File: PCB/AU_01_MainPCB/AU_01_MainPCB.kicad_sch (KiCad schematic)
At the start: 0 parts

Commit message: Created USB-C Schematic
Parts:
- added C1, C38, C39, C46, C47, C48, C49, C50, C51, C53, C54, C55, C56, C57, C58: 100nF, symbol Device:C
- added C2: 1uF, symbol Device:C
- added C40, C42, C45: 10uF, symbol Device:C_Polarized
- added C41: 10uF (Tantalum), symbol Device:C_Polarized
- added C52: 150uF, symbol Device:C_Polarized
- added CR1: SP3010-04UTG, UDFEN-10_MO229_LTF, symbol SP3010-04UTG:SP3010-04UTG
- added D1: SMAJ33CA, Diode_SMD:D_SMA, symbol Diode:SMAJ33CA
- added D11: D, symbol Device:D
- added J1: SS-53200-001, SS-53200-001:STEWART_SS-53200-001, symbol SS-53200-001:SS-53200-001
- added J6: 1-2199230-6, 1-2199230-6:TE_1-2199230-6, symbol 1-2199230-6:1-2199230-6
- added R17: 10k, symbol Device:R
- added U1: (no value), symbol Firefly_I-CORE3576Q38:I-CORE3576Q38
- added U18: SSP7903P12FR, Package_TO_SOT_SMD:SOT-223-3_TabPin2, symbol Regulator_Linear:LM317_SOT-223
- added U19: AMS1086CM3.3, TO-263DD_M_ADS, symbol AMS1086CM-3.3:AMS1086CM3.3
- added U2, U3: TPD4E02B04DQA, Package_SON:USON-10_2.5x1.0mm_P0.5mm, symbol Power_Protection:TPD4E02B04DQA
- added VR1: LM1085ISX-5.0_NOPB, LM1085ISX-5.0_NOPB:TO254P1435X464-4N, symbol LM1085ISX-5.0/NOPB:LM1085ISX-5.0_NOPB
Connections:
- new net: C49.2, U1.70 (USB3_OTG0_SSRX2N)
- new net: C51.2, U1.74 (USB3_OTG0_SSTX2P)
- new net: C46.2, U1.64 (USB3_OTG0_SSTX1P)
- new net: C53.1, U1.29 (PCIE0_REFCLKN_(OUTPUT))
- new net: C53.2, J6.53
- new net: J6.54, U1.138 (PCIE0_WAKEN_M1)
- new net: J6.52, U1.142 (PCIE0_CLKREQN_M1)
- new net: CR1.1, CR1.10, J1.15 (SCL), U1.15 (PWM2_CH0_M1)
- new net: R17.1, U1.16 (USB2_OTG0_VBUSDET)
- new net: CR1.4, CR1.7, J1.19 (HOT_PLUG_DETECT), U1.17 (PWM0_CH1_M1)
- new net: CR1.2, CR1.9, J1.16 (SDA), U1.21 (PWM2_CH1_M1)
- new net: C54.1, U1.31 (PCIE0_REFCLKP_(OUTPUT))
- new net: C55.1, U1.33 (PCIE0_RXN)
- new net: C56.1, U1.35 (PCIE0_RXP)
- new net: C57.1, U1.37 (PCIE0_TXN)
- new net: C58.1, U1.39 (PCIE0_TXP)
- new net: C38.2, U1.60 (USB3_OTG0_SSRX1P)
- new net: C39.2, U1.62 (USB3_OTG0_SSRX1N)
- new net: C47.2, U1.66 (USB3_OTG0_SSTX1N)
- new net: C48.2, U1.68 (USB3_OTG0_SSRX2P)
- new net: C50.2, U1.72 (USB3_OTG0_SSTX2N)
- new net: J1.12 (DATA3-), U1.83 (HDMI_TX_D3N), U2.5 (IO4), U2.6 (NC)
- new net: J1.10 (DATA3+), U1.85 (HDMI_TX_D3P), U2.4 (IO3), U2.7 (NC)
- new net: J1.9 (DATA0-), U1.87 (HDMI_TX_D0N), U2.2 (IO2), U2.9 (NC)
- new net: J1.7 (DATA0+), U1.89 (HDMI_TX_D0P), U2.1 (IO1), U2.10 (NC)
- new net: J1.6 (DATA1-), U1.91 (HDMI_TX_D1N), U3.5 (IO4), U3.6 (NC)
- new net: J1.4 (DATA1+), U1.93 (HDMI_TX_D1P), U3.4 (IO3), U3.7 (NC)
- new net: J1.3 (DATA2-), U1.95 (HDMI_TX_D2N), U3.2 (IO2), U3.9 (NC)
- new net: J1.1 (DATA2+), U1.97 (HDMI_TX_D2P), U3.1 (IO1), U3.10 (NC)
- new net: C56.2, J6.43
- new net: C55.2, J6.41
- new net: C58.2, J6.49
- new net: C57.2, J6.47
- new net: C54.2, J6.55
- new net 12V: C45.1, U18.2 (VO)
- new net 3V3_HIPWR: C52.1, D11.2 (A), J6.12, J6.14, J6.16, J6.18, J6.2, J6.4, J6.70, J6.72, J6.74, U19.2 (VOUT), U19.4 (OUTPUT)
- new net 3V3_O: U1.125 (VCC_3V3_S3_（OUTPUT）), U1.127 (VCC_3V3_S3_（OUTPUT）)
- new net GND: C1.2, C2.2, C40.2, C41.2, C42.2, C45.2, C52.2, CR1.3, CR1.5, CR1.6, CR1.8, D1.1 (A1), J1.11 (DATA3_SHIELD), J1.17 (DDC/CEC_GND), J1.2 (DATA2_SHIELD), J1.5 (DATA1_SHIELD), J1.8 (DATA0_SHIELD), J1.SH1 (SHIELD), J1.SH2 (SHIELD), J1.SH3 (SHIELD), J1.SH4 (SHIELD), J6.1, J6.15, J6.21, J6.27, J6.3, J6.33, J6.39, J6.45, J6.51, J6.57, J6.71, J6.73, J6.75, J6.9, J6.S1 (SHIELD), J6.S2 (SHIELD), R17.2, U1.110 (GND), U1.111 (GND), U1.112 (GND), U1.113 (GND), U1.114 (GND), U1.115 (GND), U1.116 (GND), U1.117 (GND), U1.122 (GND), U1.132 (GND), U1.143 (GND), U1.146 (GND), U1.157 (GND), U1.168 (GND), U1.169 (GND), U1.2 (GND), U1.27 (GND), U1.41 (GND), U1.44 (GND), U1.54 (GND), U1.55 (GND), U1.76 (GND), U1.77 (GND), U1.99 (GND), U18.1 (ADJ), U19.1 (GND), U2.3 (G), U2.8 (G), U3.3 (G), U3.8 (G), VR1.1 (ADJ/GND)
- new net SCL_6: U1.25 (PWM2_CH2_M1)
- new net SDA_6: U1.23 (PWM2_CH3_M1)
- new net SYS_5V: C1.1, C2.1, C41.1, D1.2 (A2), D11.1 (K), J1.18 (+5V), U1.101 (VCC5V0_SYS_S5), U1.102 (VCC5V0_SYS_S5), U1.103 (VCC5V0_SYS_S5), U1.104 (VCC5V0_SYS_S5), U1.105 (VCC5V0_SYS_S5), U1.106 (VCC5V0_SYS_S5), U1.107 (VCC5V0_SYS_S5), U1.108 (VCC5V0_SYS_S5), U1.109 (VCC5V0_SYS_S5), U19.3 (VIN), VR1.2 (OUTPUT_2), VR1.4 (OUTPUT_4)
- new net USBC0_DN: U1.48 (USB2_OTG1_DM)
- new net USBC0_DP: U1.46 (USB2_OTG1_DP)
- new net USBC1_DN_O: U1.52 (USB2_OTG0_DM)
- new net USBC1_DP_O: U1.50 (USB2_OTG0_DP)
- new net USBC1_SSRX1N: C47.1
- new net USBC1_SSRX1P: C46.1
- new net USBC1_SSRX2N: C50.1
- new net USBC1_SSRX2P: C51.1
- new net USBC1_SSTX1N: C39.1
- new net USBC1_SSTX1P: C38.1
- new net USBC1_SSTX2N: C49.1
- new net USBC1_SSTX2P: C48.1
- new net USBC1_SW_EN: U1.6 (CAN1_TX_M2)
- new net USBC_1_INT: U1.4 (SPDIF_RX0_M0)
- new net VSYS: C40.1, C42.1, U18.3 (VI), VR1.3 (INPUT)
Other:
- added sheet AU_01 Audio System (AU_01_AudioSystem.kicad_sch)
- added sheet AU_01 Battery Circuit (AU_01_BatteryCircuit.kicad_sch)
- added sheet AU_01 USB-C Ports (AU_01_USBC_Ports.kicad_sch)

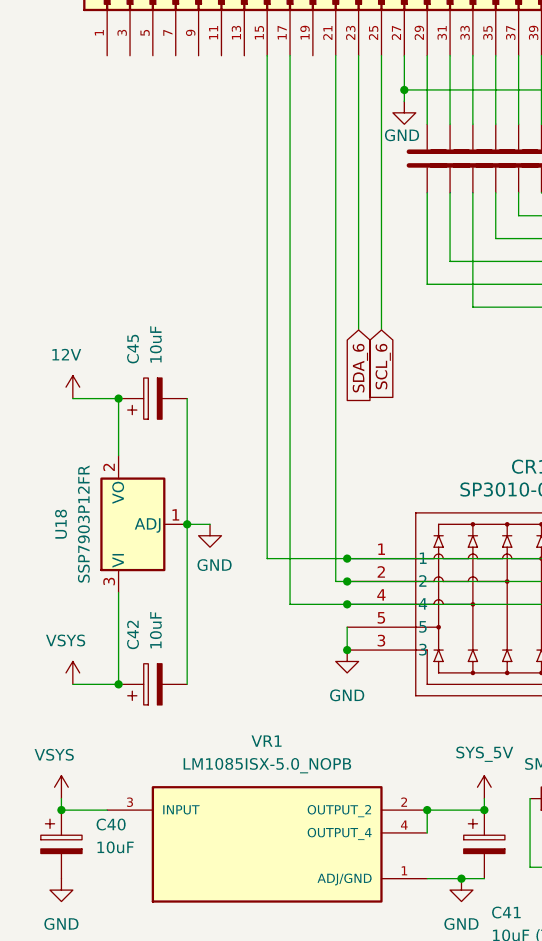
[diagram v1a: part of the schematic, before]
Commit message: Audio, Battery Schematic, added Journal
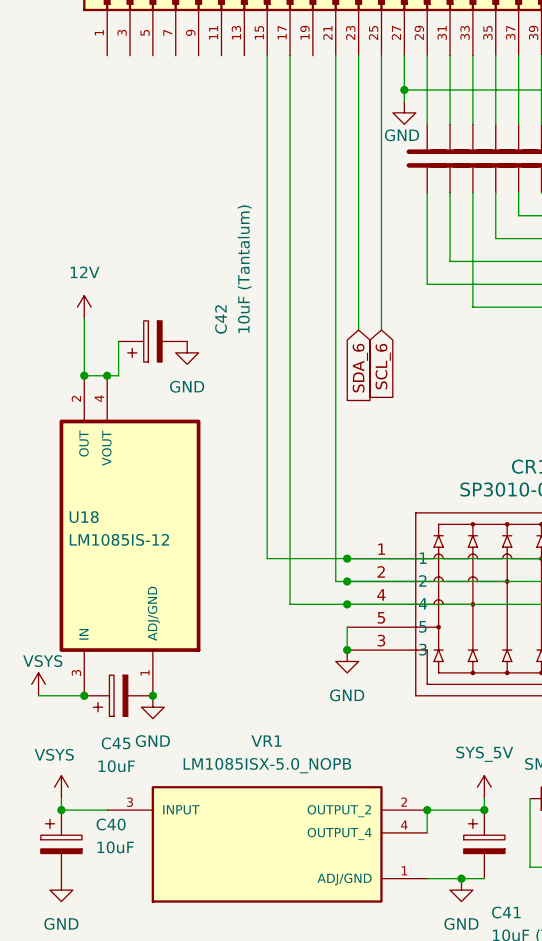
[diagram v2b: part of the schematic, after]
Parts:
- removed U18: SSP7903P12FR, Package_TO_SOT_SMD:SOT-223-3_TabPin2, symbol Regulator_Linear:LM317_SOT-223
- added U18: LM1085IS-12, LM1085IS-12:TO254P1524X483-4N, symbol LM1085IS-12/NOPB:LM1085IS-12
- C42: value 10uF -> 10uF (Tantalum)
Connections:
- net 12V: now also C42.1, U18.2 (OUT), U18.4 (VOUT); no longer C45.1
- net GND: now also U18.1 (ADJ/GND)
- net VSYS: now also C45.1, U18.3 (IN); no longer C42.1
